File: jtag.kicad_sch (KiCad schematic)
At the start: 1 part, among them J3 878321420

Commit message: more stuff!
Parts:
- J3: footprint CONN_87832-1420_MOL -> 878321420:CONN_87832-1420_MOL
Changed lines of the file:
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@@
 			)
 		)
-		(property "Footprint" "CONN_87832-1420_MOL"
+		(property "Footprint" "878321420:CONN_87832-1420_MOL"
 			(at 144.78 77.47 0)
 			(effects

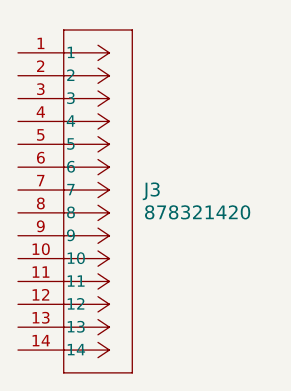
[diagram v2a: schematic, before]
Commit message: added a lot of stuff
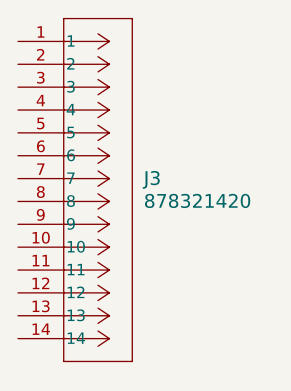
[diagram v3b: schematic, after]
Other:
- moved on the sheet: J3
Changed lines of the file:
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@@
 	(symbol
 		(lib_id "878321420:878321420")
-		(at 144.78 77.47 0)
+		(at 144.78 76.2 0)
 		(unit 1)
 		(exclude_from_sim no)
@@
 		(fields_autoplaced yes)
 		(property "Reference" "J3"
-			(at 158.75 92.7099 0)
+			(at 158.75 91.4399 0)
 			(effects
 				(font
@@
 		)
 		(property "Value" "878321420"
-			(at 158.75 95.2499 0)
+			(at 158.75 93.9799 0)
 			(effects
 				(font
@@
 		)
 		(property "Footprint" "878321420:CONN_87832-1420_MOL"
-			(at 144.78 77.47 0)
+			(at 144.78 76.2 0)
 			(effects
 				(font
@@
 		)
 		(property "Datasheet" "878321420"
-			(at 144.78 77.47 0)
+			(at 144.78 76.2 0)
 			(effects
 				(font
@@
 		)
 		(property "Description" ""
-			(at 144.78 77.47 0)
+			(at 144.78 76.2 0)
 			(effects
 				(font
